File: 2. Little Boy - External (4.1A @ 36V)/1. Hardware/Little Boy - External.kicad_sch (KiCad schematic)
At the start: 80 parts, among them J1 TESTPOINT, J10 MOT_B, J11 MOT_A, J12 TESTPOINT, J13 Control_In, J14 Control_In, J15 Conn_01x06_MountingPin, J16 Conn_01x06_MountingPin, J17 TESTPOINT, J2 TESTPOINT, J3 TESTPOINT, J4 Prog_IN, J5 Conn_01x06_MountingPin, J6 TESTPOINT, J7 TESTPOINT, J8 Power_In, J9 Power_In, U1 STM32G0B1CBTx, U2 LMR33630CDDA, U3 TJA1051T-3, U4 TLV76733DRVx, U5 MA730, U6 W25Q128JVS, U7 DRV8251DDAR, U8 AS5600-ASOT, Y1 25 MHz

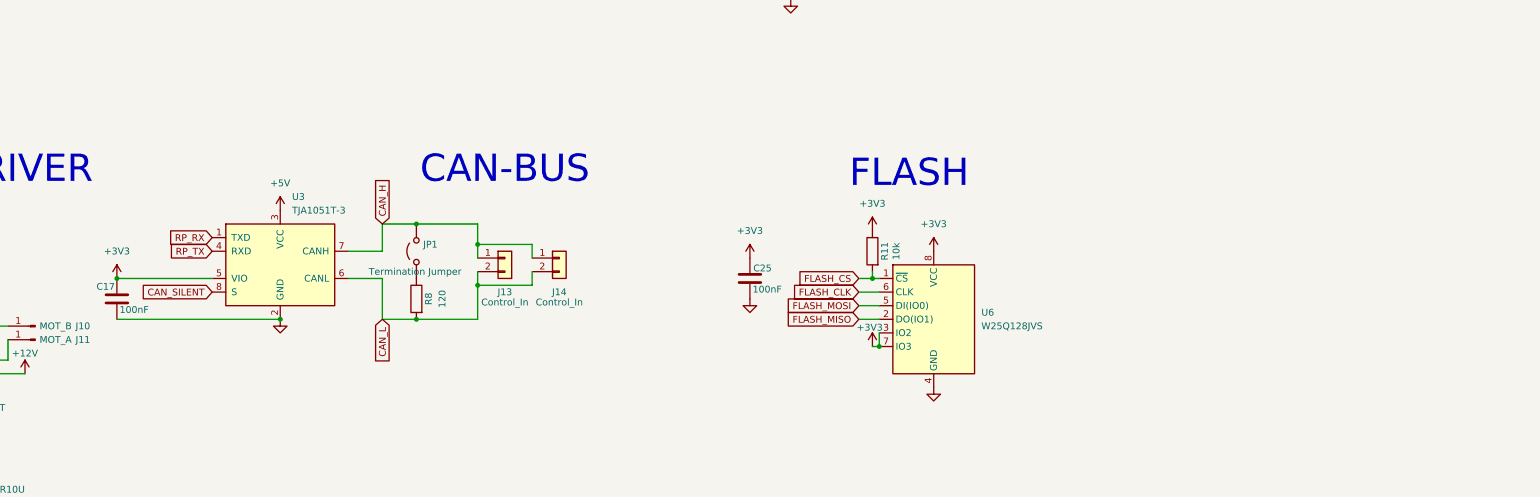
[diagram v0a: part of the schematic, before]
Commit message: V0.4
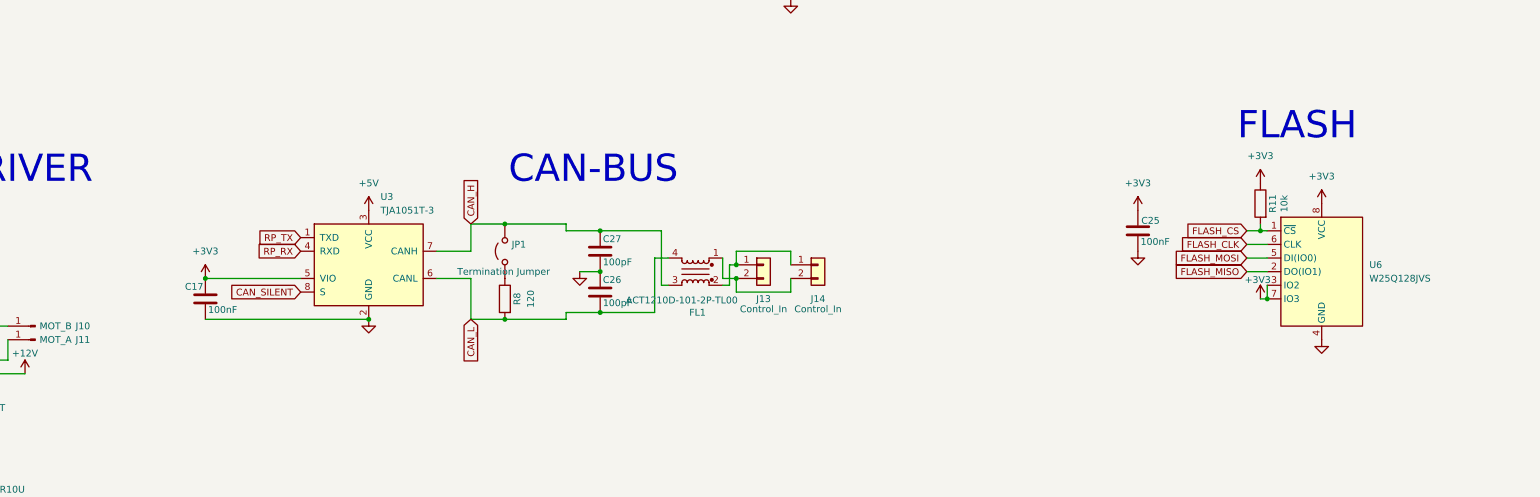
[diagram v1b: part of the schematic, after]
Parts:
- added C26, C27: 100pF, Capacitor_SMD:C_0402_1005Metric, symbol Device:C
- added FL1: ACT1210D-101-2P-TL00, _custom:ACT1210D1012PTL00, symbol Device:Filter_EMI_LL_1423
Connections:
- net CAN_H: now also C27.1, FL1.3; no longer J13.1 (Pin_1), J14.1 (Pin_1)
- net CAN_L: now also C26.2, FL1.4; no longer J13.2 (Pin_2), J14.2 (Pin_2)
- net GND: now also C26.1, C27.2
- net RP_RX: now also U3.4 (RXD); no longer U3.1 (TXD)
- net RP_TX: now also U3.1 (TXD); no longer U3.4 (RXD)
- new net: FL1.2, J13.1 (Pin_1), J14.1 (Pin_1)
- new net: FL1.1, J13.2 (Pin_2), J14.2 (Pin_2)
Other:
- moved on the sheet: C17, C25, J13, J14, JP1, R11, R8, U3, U6
